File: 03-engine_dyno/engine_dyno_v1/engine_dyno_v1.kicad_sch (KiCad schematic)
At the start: 0 parts

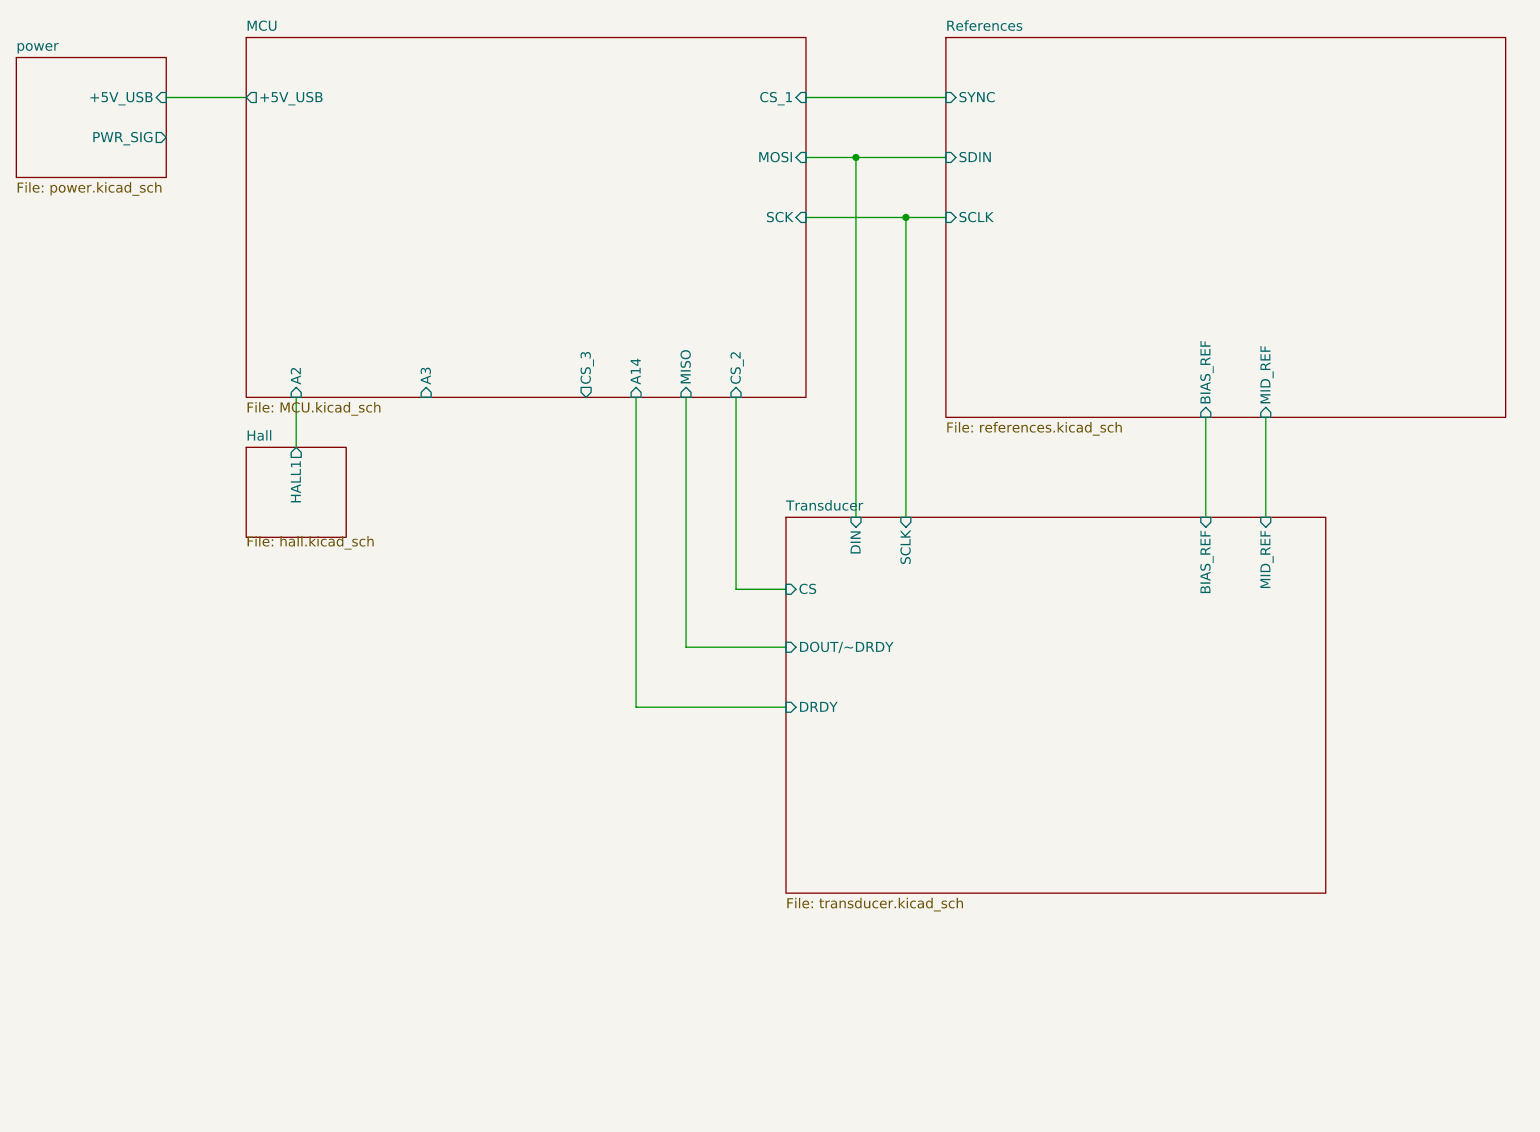
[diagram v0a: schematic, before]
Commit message: clean up
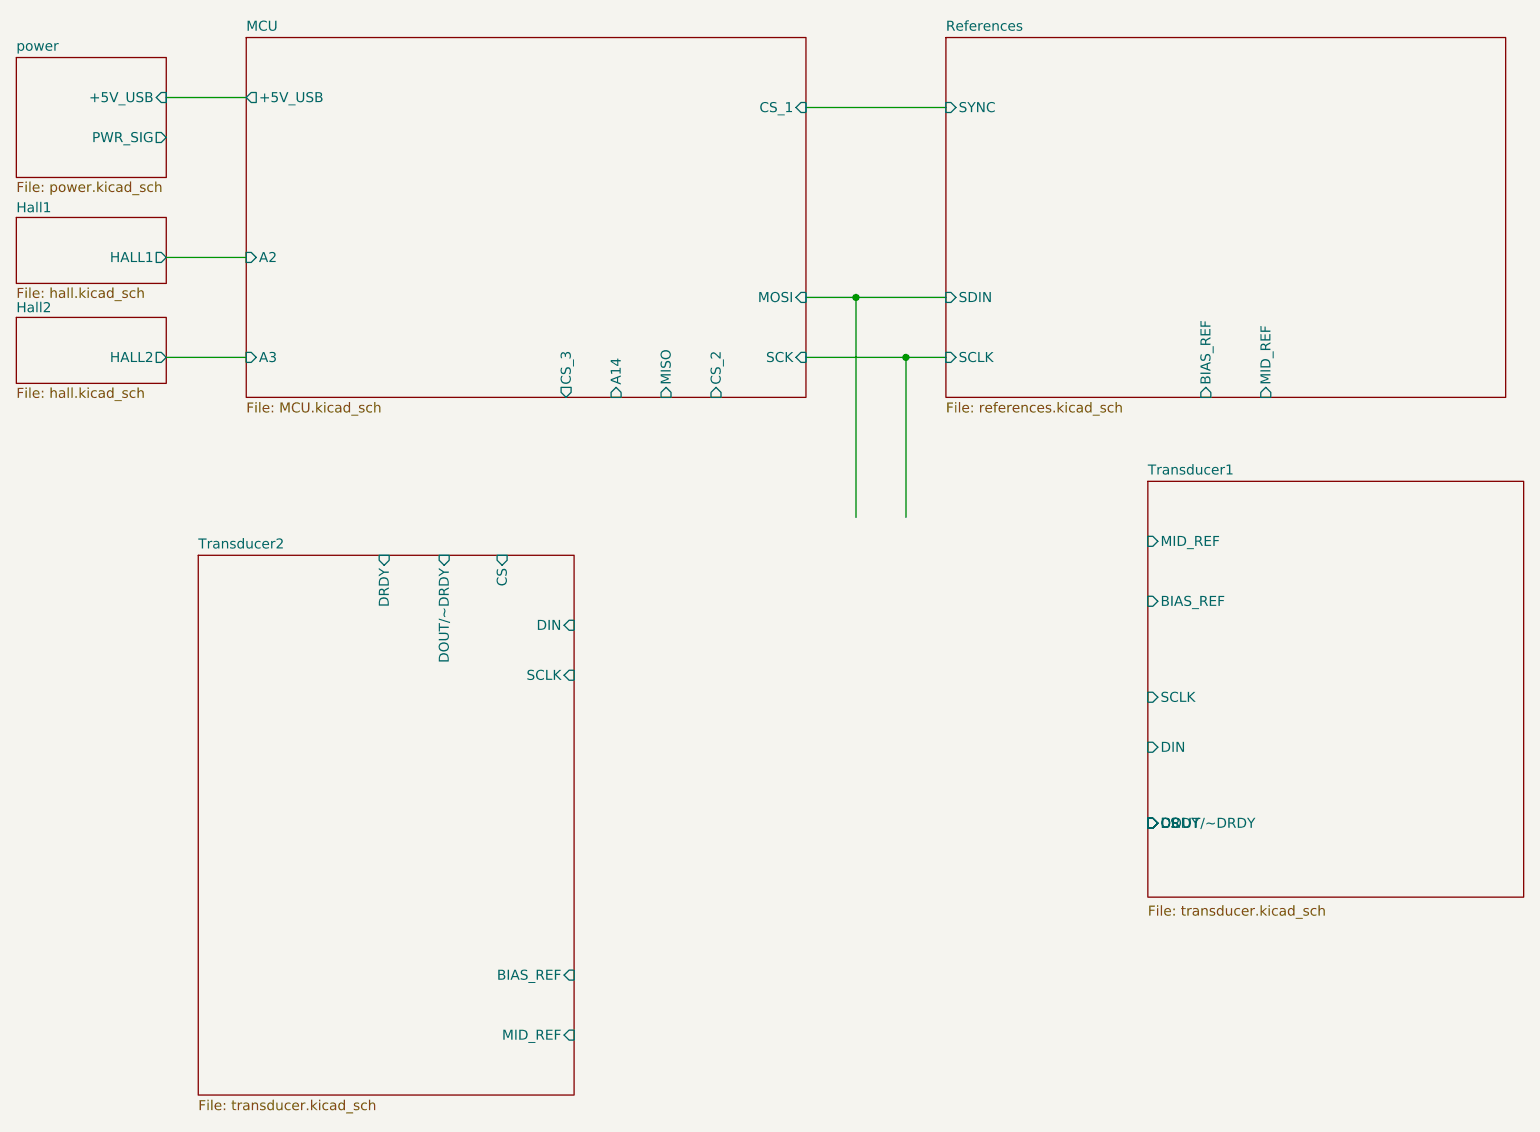
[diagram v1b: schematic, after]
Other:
- sheet Hall renamed Hall1
- sheet Transducer renamed Transducer1
- added sheet Hall2 (hall.kicad_sch)
- added sheet Transducer2 (transducer.kicad_sch)
